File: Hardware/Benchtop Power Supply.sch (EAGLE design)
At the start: 20 parts, among them J1 ATX24RH

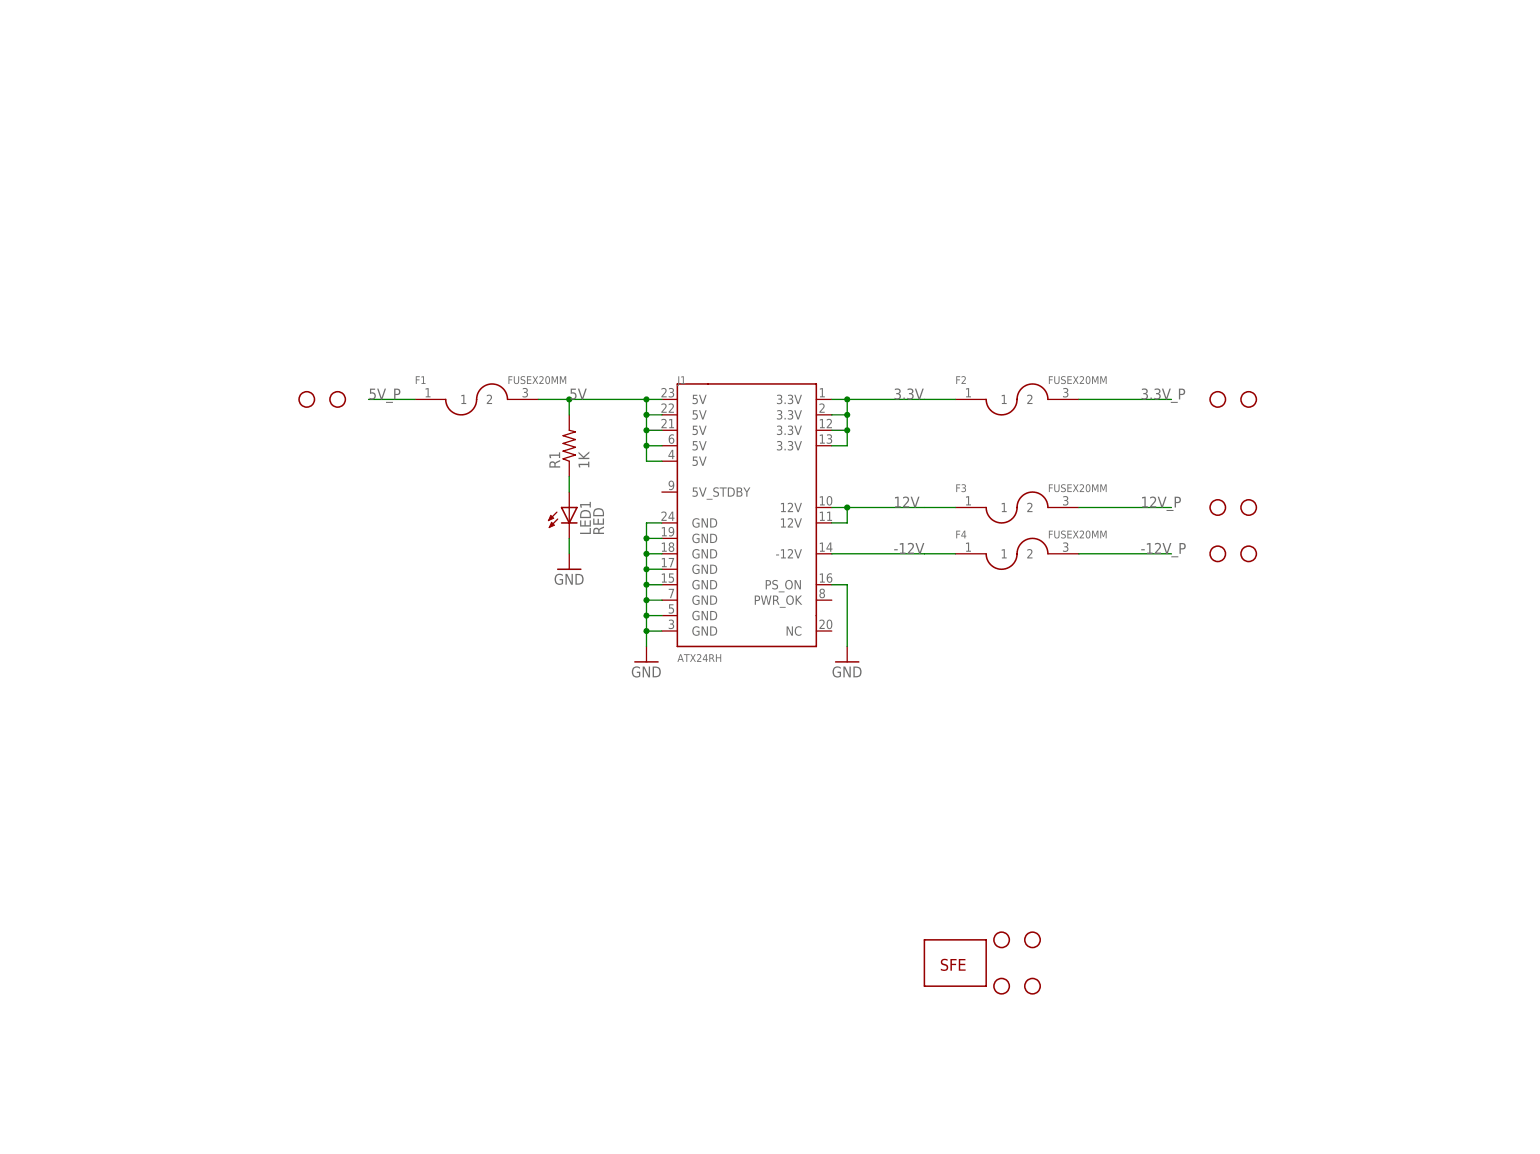
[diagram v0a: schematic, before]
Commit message: Midway hardware changes
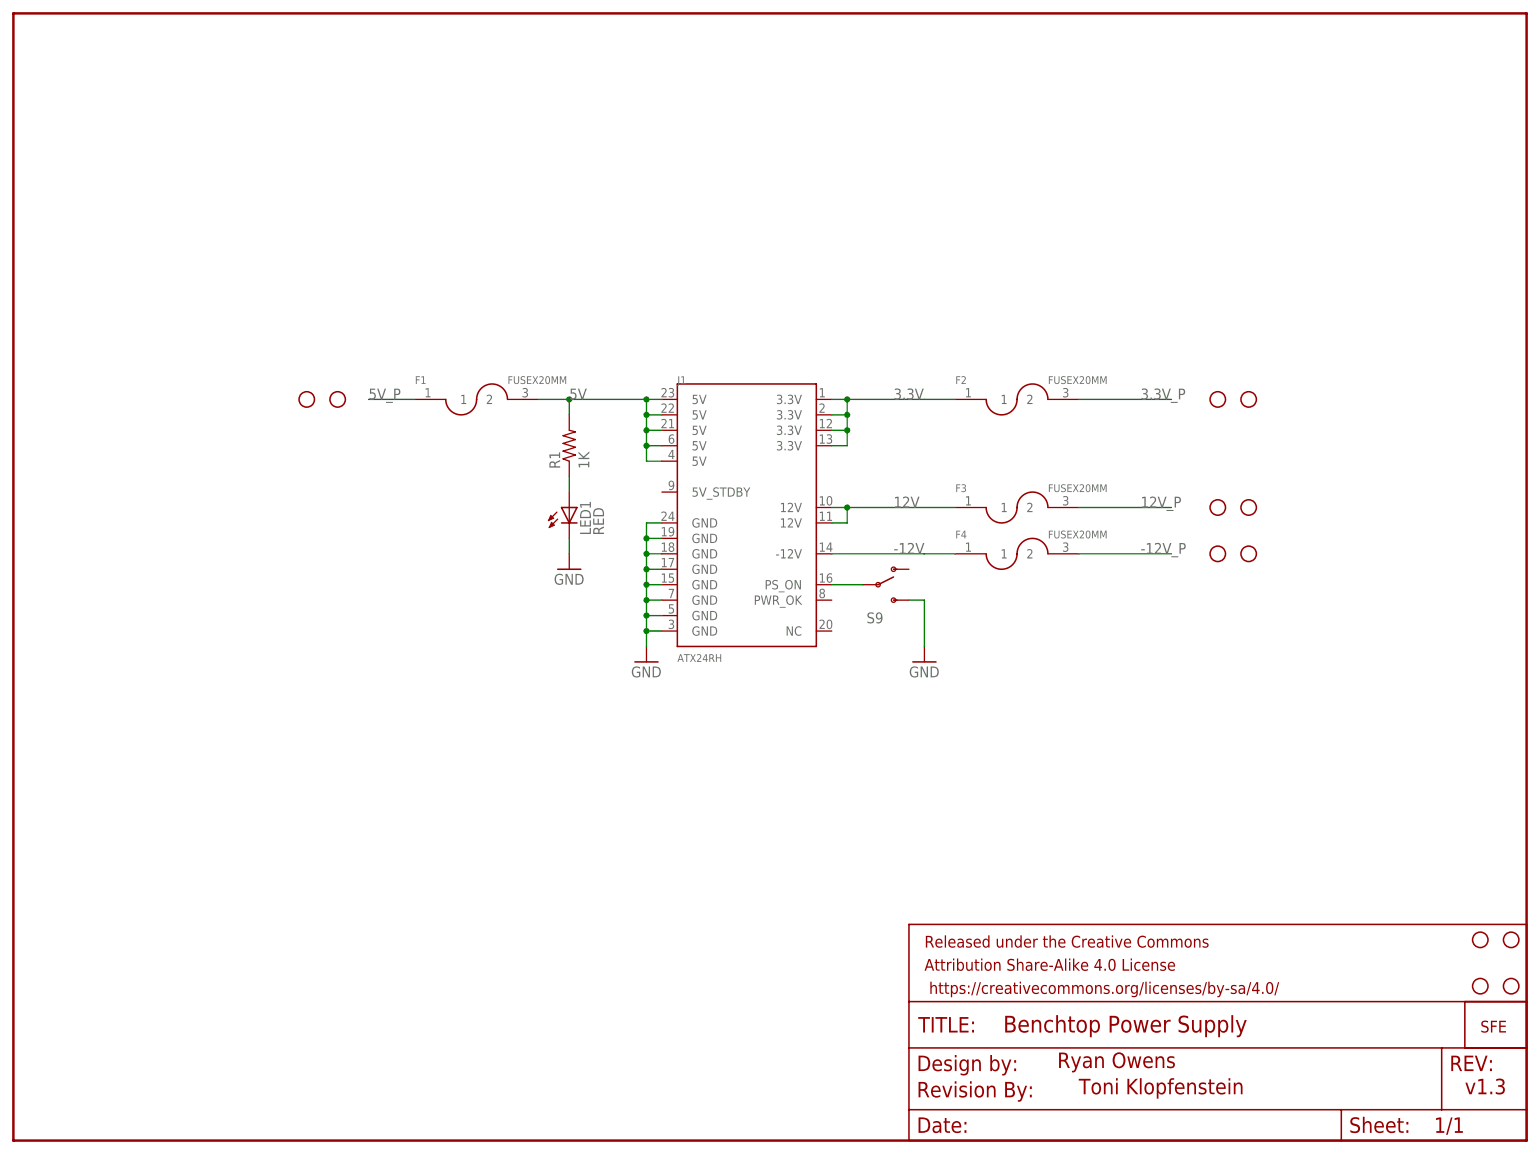
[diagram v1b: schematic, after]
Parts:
- added FRAME1: FRAME-LETTER, SparkFun-Aesthetics:FRAME-LETTER
- added S9: (no value), SparkFun-Electromechanical:SWITCH-SPDTKIT
- added U$1: REVISION, SparkFun-Aesthetics:REVISION
- J1: device SparkFun:ATX24RH -> SparkFun-Connectors:ATX24RH
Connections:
- new net N$2: J1.PS_ON, S9.P
- net GND: now also S9.S; no longer J1.PS_ON
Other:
- note added: "Ryan Owens"
- note added: "Toni Klopfenstein"
- note added: "v1.3"
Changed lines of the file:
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@@
 <layer number="106" name="bPlate" color="7" fill="1" visible="yes" active="yes"/>
 <layer number="107" name="Crop" color="7" fill="1" visible="yes" active="yes"/>
+<layer number="108" name="tplace-old" color="10" fill="1" visible="yes" active="yes"/>
+<layer number="109" name="ref-old" color="11" fill="1" visible="yes" active="yes"/>
+<layer number="110" name="fp0" color="7" fill="1" visible="yes" active="yes"/>
+<layer number="111" name="LPC17xx" color="7" fill="1" visible="yes" active="yes"/>
+<layer number="112" name="tSilk" color="7" fill="1" visible="yes" active="yes"/>
+<layer number="113" name="IDFDebug" color="4" fill="1" visible="yes" active="yes"/>
 <layer number="116" name="Patch_BOT" color="9" fill="4" visible="yes" active="yes"/>
 <layer number="121" name="_tsilk" color="7" fill="1" visible="yes" active="yes"/>
 <layer number="122" name="_bsilk" color="7" fill="1" visible="yes" active="yes"/>
+<layer number="123" name="tTestmark" color="7" fill="1" visible="yes" active="yes"/>
+<layer number="124" name="bTestmark" color="7" fill="1" visible="yes" active="yes"/>
+<layer number="125" name="_tNames" color="7" fill="1" visible="yes" active="yes"/>
+<layer number="126" name="_bNames" color="7" fill="1" visible="yes" active="yes"/>
+<layer number="127" name="_tValues" color="7" fill="1" visible="yes" active="yes"/>
+<layer number="128" name="_bValues" color="7" fill="1" visible="yes" active="yes"/>
+<layer number="131" name="tAdjust" color="7" fill="1" visible="yes" active="yes"/>
+<layer number="132" name="bAdjust" color="7" fill="1" visible="yes" active="yes"/>
+<layer number="144" name="Drill_legend" color="7" fill="1" visible="yes" active="yes"/>
 <layer number="151" name="HeatSink" color="7" fill="1" visible="yes" active="yes"/>
+<layer number="152" name="_bDocu" color="7" fill="1" visible="yes" active="yes"/>
+<layer number="199" name="Contour" color="7" fill="1" visible="yes" active="yes"/>
 <layer number="200" name="200bmp" color="1" fill="10" visible="yes" active="yes"/>
 <layer number="201" name="201bmp" color="2" fill="10" visible="yes" active="yes"/>
@@
 <layer number="207" name="207bmp" color="8" fill="10" visible="yes" active="yes"/>
 <layer number="208" name="208bmp" color="9" fill="10" visible="yes" active="yes"/>
+<layer number="209" name="209bmp" color="7" fill="1" visible="yes" active="yes"/>
+<layer number="210" name="210bmp" color="7" fill="1" visible="yes" active="yes"/>
+<layer number="211" name="211bmp" color="7" fill="1" visible="yes" active="yes"/>
+<layer number="212" name="212bmp" color="7" fill="1" visible="yes" active="yes"/>
+<layer number="213" name="213bmp" color="7" fill="1" visible="yes" active="yes"/>
+<layer number="214" name="214bmp" color="7" fill="1" visible="yes" active="yes"/>
+<layer number="215" name="215bmp" color="7" fill="1" visible="yes" active="yes"/>
+<layer number="216" name="216bmp" color="7" fill="1" visible="yes" active="yes"/>
+<layer number="217" name="217bmp" color="18" fill="1" visible="no" active="no"/>
+<layer number="218" name="218bmp" color="19" fill="1" visible="no" active="no"/>
+<layer number="219" name="219bmp" color="20" fill="1" visible="no" active="no"/>
+<layer number="220" name="220bmp" color="21" fill="1" visible="no" active="no"/>
+<layer number="221" name="221bmp" color="22" fill="1" visible="no" active="no"/>
+<layer number="222" name="222bmp" color="23" fill="1" visible="no" active="no"/>
+<layer number="223" name="223bmp" color="24" fill="1" visible="no" active="no"/>
+<layer number="224" name="224bmp" color="25" fill="1" visible="no" active="no"/>
+<layer number="248" name="Housing" color="7" fill="1" visible="yes" active="yes"/>
+<layer number="249" name="Edge" color="7" fill="1" visible="yes" active="yes"/>
 <layer number="250" name="Descript" color="3" fill="1" visible="no" active="no"/>
 <layer number="251" name="SMDround" color="12" fill="11" visible="no" active="no"/>
@@
 </classes>
 <parts>
-<part name="FRAME1" library="SparkFun" deviceset="FRAME-LETTER" device=""/>
+<part name="FRAME1" library="SparkFun-Aesthetics" deviceset="FRAME-LETTER" device=""/>
 <part name="JP1" library="SparkFun" deviceset="LOGO-SFE" device="NEW"/>
 <part name="JP2" library="SparkFun" deviceset="STAND-OFF" device=""/>
@@
 <part name="JP4" library="SparkFun" deviceset="STAND-OFF" device=""/>
 <part name="JP5" library="SparkFun" deviceset="STAND-OFF" device=""/>
-<part name="J1" library="SparkFun" deviceset="ATX24" device="RH"/>
+<part name="J1" library="SparkFun-Connectors" deviceset="ATX24" device="RH"/>
 <part name="GND1" library="SparkFun" deviceset="GND" device=""/>
 <part name="GND2" library="SparkFun" deviceset="GND" device=""/>
@@
 <part name="S7" library="SparkFun" deviceset="BINDING_POST" device=""/>
 <part name="S8" library="SparkFun" deviceset="BINDING_POST" device=""/>
+<part name="S9" library="SparkFun-Electromechanical" deviceset="SWITCH-SPDT" device="KIT"/>
+<part name="U$1" library="SparkFun-Aesthetics" deviceset="REVISION" device=""/>
 </parts>
 <sheets>
 <sheet>
 <plain>
+<text x="171.704" y="11.938" size="2.54" layer="94">Ryan Owens</text>
+<text x="175.26" y="7.62" size="2.54" layer="94">Toni Klopfenstein</text>
+<text x="238.76" y="7.62" size="2.54" layer="94">v1.3</text>
 </plain>
 <instances>
 <instance part="FRAME1" gate="G$1" x="0" y="0"/>
 <instance part="FRAME1" gate="G$2" x="147.32" y="0"/>
-<instance part="JP1" gate="G$1" x="152.4" y="27.94"/>
-<instance part="JP2" gate="G$1" x="162.56" y="33.02"/>
-<instance part="JP3" gate="G$1" x="162.56" y="25.4"/>
-<instance part="JP4" gate="G$1" x="167.64" y="33.02"/>
-<instance part="JP5" gate="G$1" x="167.64" y="25.4"/>
+<instance part="JP1" gate="G$1" x="241.3" y="17.78"/>
+<instance part="JP2" gate="G$1" x="246.38" y="33.02"/>
+<instance part="JP3" gate="G$1" x="241.3" y="25.4"/>
+<instance part="JP4" gate="G$1" x="241.3" y="33.02"/>
+<instance part="JP5" gate="G$1" x="246.38" y="25.4"/>
 <instance part="J1" gate="G$1" x="121.92" y="104.14"/>
 <instance part="GND1" gate="1" x="104.14" y="78.74"/>
-<instance part="GND2" gate="1" x="137.16" y="78.74"/>
+<instance part="GND2" gate="1" x="149.86" y="78.74"/>
 <instance part="F1" gate="G$1" x="76.2" y="121.92"/>
 <instance part="F2" gate="G$1" x="165.1" y="121.92"/>
@@
 <instance part="S7" gate="G$1" x="53.34" y="121.92"/>
 <instance part="S8" gate="G$1" x="48.26" y="121.92"/>
+<instance part="S9" gate="1" x="142.24" y="91.44"/>
+<instance part="U$1" gate="G$1" x="148.59" y="7.112"/>
 </instances>
 <busses>
@@
 <nets>
 <net name="GND" class="0">
-<segment>
-<wire x1="134.62" y1="91.44" x2="137.16" y2="91.44" width="0.1524" layer="91"/>
-<wire x1="137.16" y1="91.44" x2="137.16" y2="81.28" width="0.1524" layer="91"/>
-<pinref part="J1" gate="G$1" pin="PS_ON"/>
-<pinref part="GND2" gate="1" pin="GND"/>
-</segment>
 <segment>
 <wire x1="106.68" y1="83.82" x2="104.14" y2="83.82" width="0.1524" layer="91"/>
@@
 <pinref part="LED1" gate="G$1" pin="C"/>
 </segment>
+<segment>
+<pinref part="S9" gate="1" pin="S"/>
+<wire x1="147.32" y1="88.9" x2="149.86" y2="88.9" width="0.2032" layer="91"/>
+<wire x1="149.86" y1="88.9" x2="149.86" y2="81.28" width="0.2032" layer="91"/>
+<pinref part="GND2" gate="1" pin="GND"/>
+</segment>
 </net>
 <net name="5V" class="0">
@@
 </segment>
 </net>
+<net name="N$2" class="0">
+<segment>
+<pinref part="J1" gate="G$1" pin="PS_ON"/>
+<pinref part="S9" gate="1" pin="P"/>
+<wire x1="134.62" y1="91.44" x2="139.7" y2="91.44" width="0.2032" layer="91"/>
+</segment>
+</net>
